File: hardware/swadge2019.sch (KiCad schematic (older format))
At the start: 48 parts, among them P1 PGM, P10 CONN_1, P11 CONN_1, P12 CONN_1, P13 CONN_1, P2 USBMicroB-10118192-0001LF, P3 SAO, P4 CONN_1, P6 CONN_1, P7 CONN_1, P8 CONN_1, P9 CONN_1, SW1 B, SW2 A, SW3 MODE, SW7 SWITCH_INV, U1 OPAMP_MCP6001T, U2 AP1117SOT223, Y1 Mic

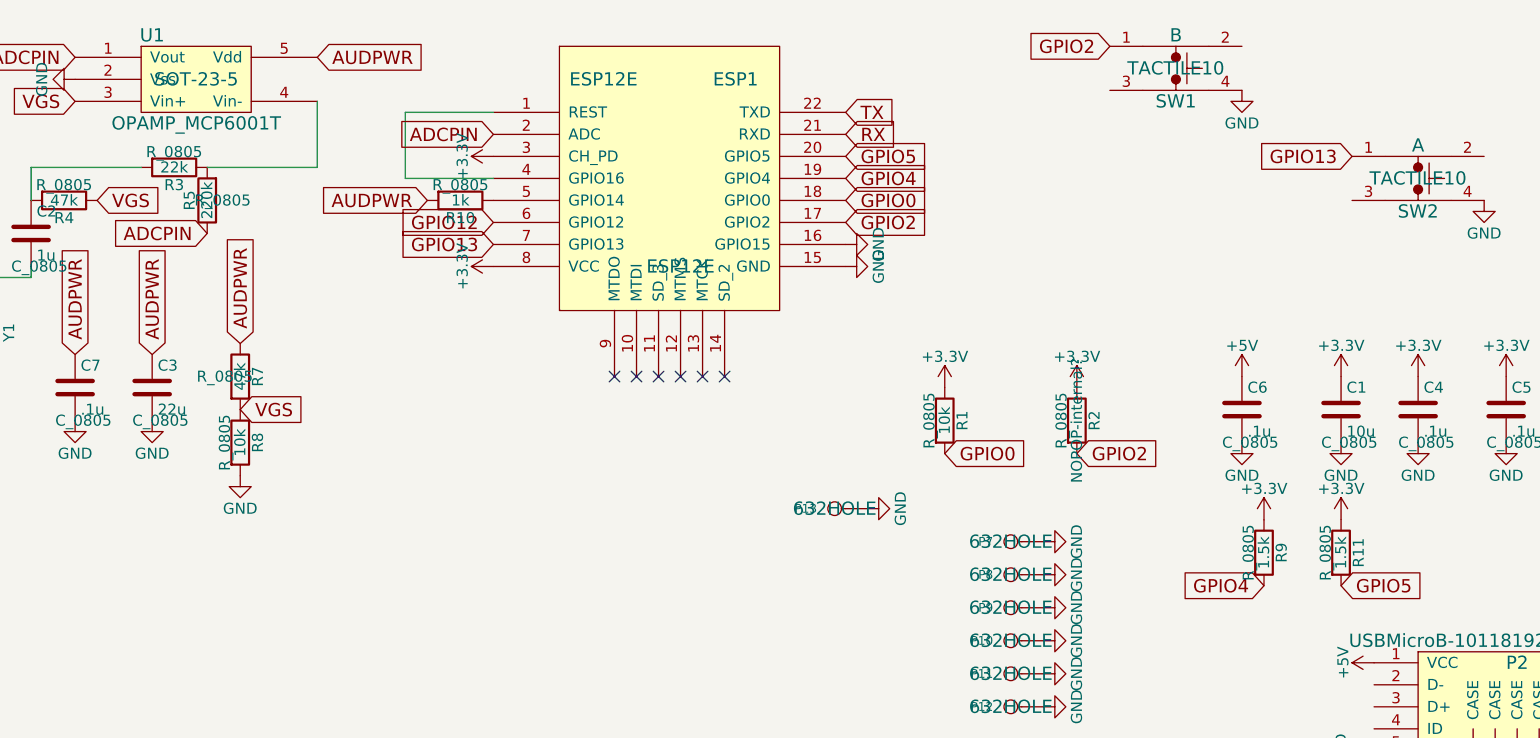
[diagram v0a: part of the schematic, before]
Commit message: update design
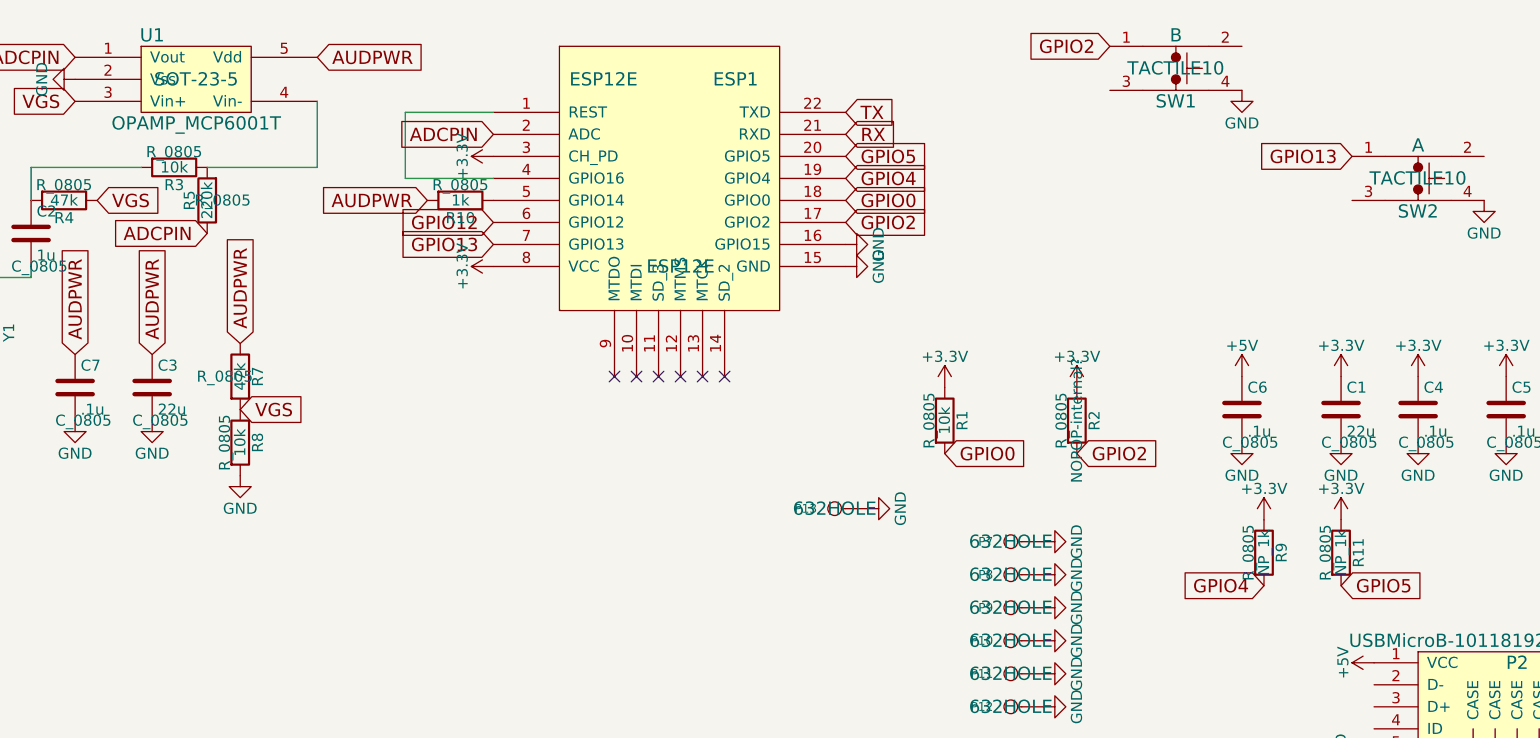
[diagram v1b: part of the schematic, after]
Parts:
- C1: value 10u -> 22u
- R11, R9: value 1.5k -> NP_1k
- R3: value 22k -> 10k
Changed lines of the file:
@@
 P 7000 3150
 F 0 "C1" H 7025 3250 50  0000 L CNN
-F 1 "10u" H 7025 3050 50  0000 L CNN
+F 1 "22u" H 7025 3050 50  0000 L CNN
 F 2 "C_0805" H 7038 3000 50  0000 C CNN
 F 3 "" H 7000 3150 50  0000 C CNN
@@
 P 1700 2050
 F 0 "R3" V 1780 2050 50  0000 C CNN
-F 1 "22k" V 1700 2050 50  0000 C CNN
+F 1 "10k" V 1700 2050 50  0000 C CNN
 F 2 "R_0805" V 1630 2050 50  0000 C CNN
 F 3 "" H 1700 2050 50  0000 C CNN
@@
 P 6650 3800
 F 0 "R9" V 6730 3800 50  0000 C CNN
-F 1 "1.5k" V 6650 3800 50  0000 C CNN
+F 1 "NP_1k" V 6650 3800 50  0000 C CNN
 F 2 "R_0805" V 6580 3800 50  0000 C CNN
 F 3 "" H 6650 3800 50  0000 C CNN
@@
 P 7000 3800
 F 0 "R11" V 7080 3800 50  0000 C CNN
-F 1 "1.5k" V 7000 3800 50  0000 C CNN
+F 1 "NP_1k" V 7000 3800 50  0000 C CNN
 F 2 "R_0805" V 6930 3800 50  0000 C CNN
 F 3 "" H 7000 3800 50  0000 C CNN
